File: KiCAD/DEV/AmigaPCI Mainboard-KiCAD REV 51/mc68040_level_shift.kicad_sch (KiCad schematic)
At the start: 27 parts, among them U231 74LVC08, U802 SN74LVC16T245DLR, U803 SN74LVC16T245DLR, U804 SN74LVC16T245DLR, U805 SN74LVC16T245DLR, U806 74LVC245, U807 74LVC245, U808 74LVC245, U809 74LVC245, U810 74LVC16646

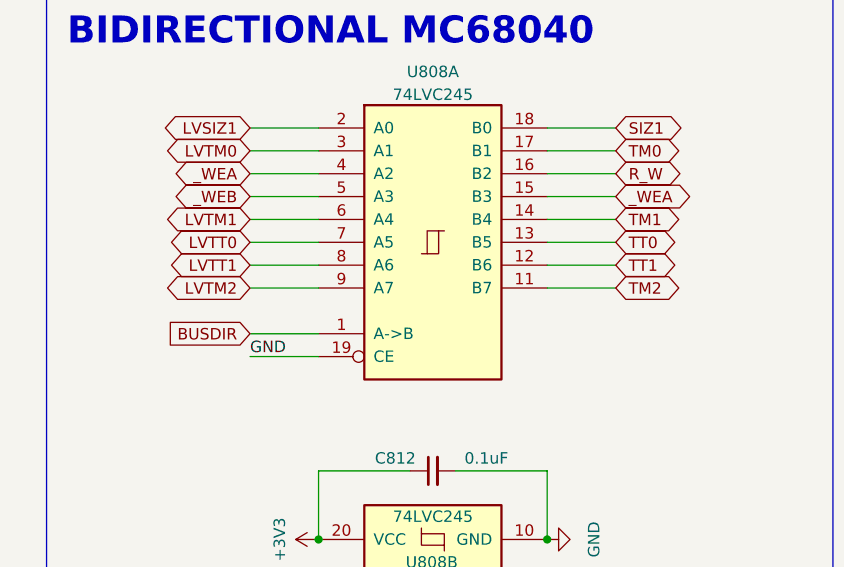
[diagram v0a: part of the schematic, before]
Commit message: Amiga PCI Rev 5.1 Work
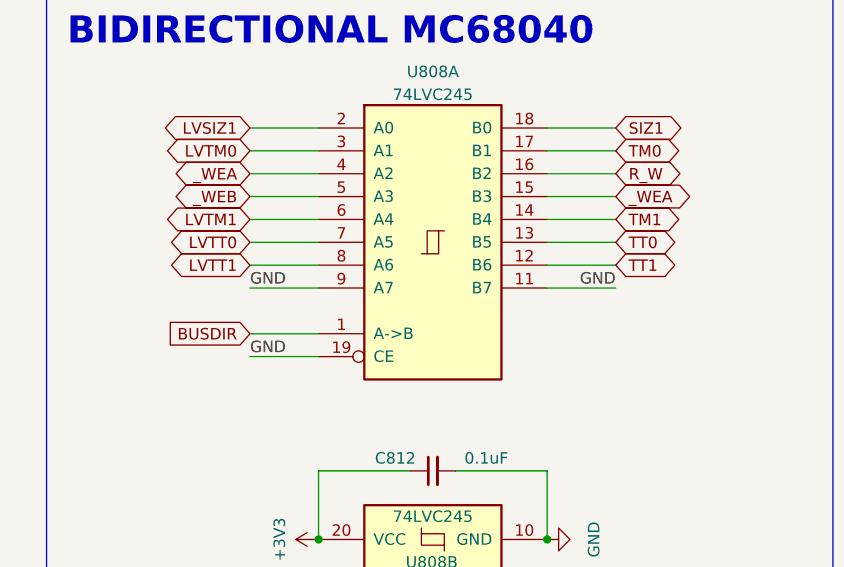
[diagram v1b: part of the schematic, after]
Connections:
- net LVTM2 is gone; now on net GND: U808.9 (A7)
- net TM2 is gone; now on net GND: U808.11 (B7)
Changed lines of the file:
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@@
 	(title_block
 		(title "AMIGA PCI")
-		(date "2025-03-31")
+		(date "2025-04-01")
 		(rev "5.1")
 	)
@@
 		)
 	)
+	(label "GND"
+		(at 234.95 170.18 0)
+		(effects
+			(font
+				(size 1.27 1.27)
+			)
+			(justify left bottom)
+		)
+	)
 	(label "UDB5"
 		(at 336.55 85.09 0)
@@
 		)
 	)
+	(label "GND"
+		(at 275.59 170.18 180)
+		(effects
+			(font
+				(size 1.27 1.27)
+			)
+			(justify right bottom)
+		)
+	)
 	(label "LVA29"
 		(at 120.65 157.48 0)
@@
 		)
 	)
-	(global_label "TM2"
-		(shape bidirectional)
-		(at 275.59 170.18 0)
-		(fields_autoplaced yes)
-		(effects
-			(font
-				(size 1.27 1.27)
-			)
-			(justify left)
-		)
-		(property "Intersheetrefs" "${INTERSHEET_REFS}"
-			(at 283.315 170.18 0)
-			(effects
-				(font
-					(size 1.27 1.27)
-				)
-				(justify left)
-			)
-		)
-	)
 	(global_label "DMALATCH"
 		(shape input)
@@
 			(effects
 				(font
-					(size 1.27 1.27)
-				)
-				(justify right)
-			)
-		)
-	)
-	(global_label "LVTM2"
-		(shape bidirectional)
-		(at 234.95 170.18 180)
-		(fields_autoplaced yes)
-		(effects
-			(font
-				(size 1.27 1.27)
-			)
-			(justify right)
-		)
-		(property "Intersheetrefs" "${INTERSHEET_REFS}"
-			(at 225.1083 170.18 0)
-			(effects
-				(font

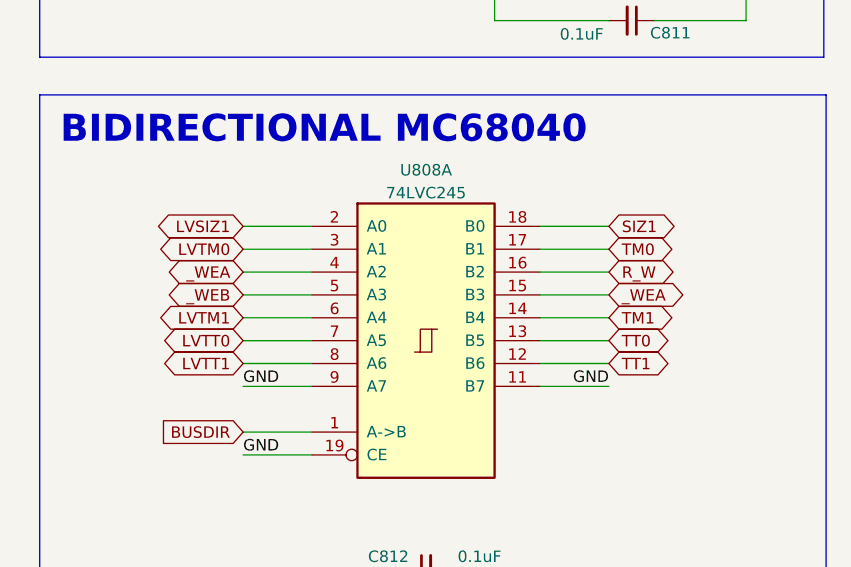
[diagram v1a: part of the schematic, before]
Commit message: APCI Rev 5.1 Work
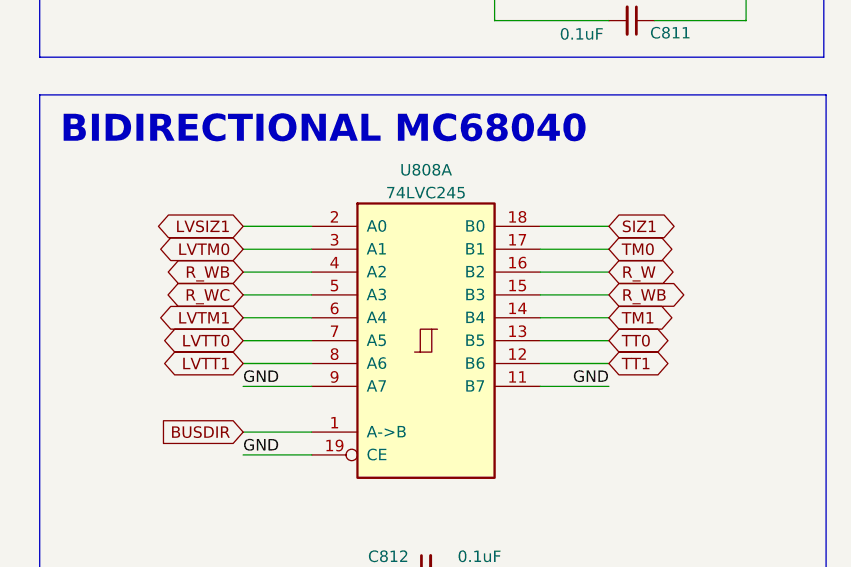
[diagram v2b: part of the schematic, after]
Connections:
- net _WEA renamed R_WB
- net _WEB renamed R_WC
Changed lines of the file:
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@@
 		)
 	)
-	(global_label "_WEB"
+	(global_label "R_WC"
 		(shape bidirectional)
 		(at 234.95 160.02 180)
@@
 		)
 	)
-	(global_label "_WEA"
+	(global_label "R_WB"
 		(shape bidirectional)
 		(at 275.59 160.02 0)
@@
 		)
 	)
-	(global_label "_WEA"
+	(global_label "R_WB"
 		(shape bidirectional)
 		(at 234.95 157.48 180)

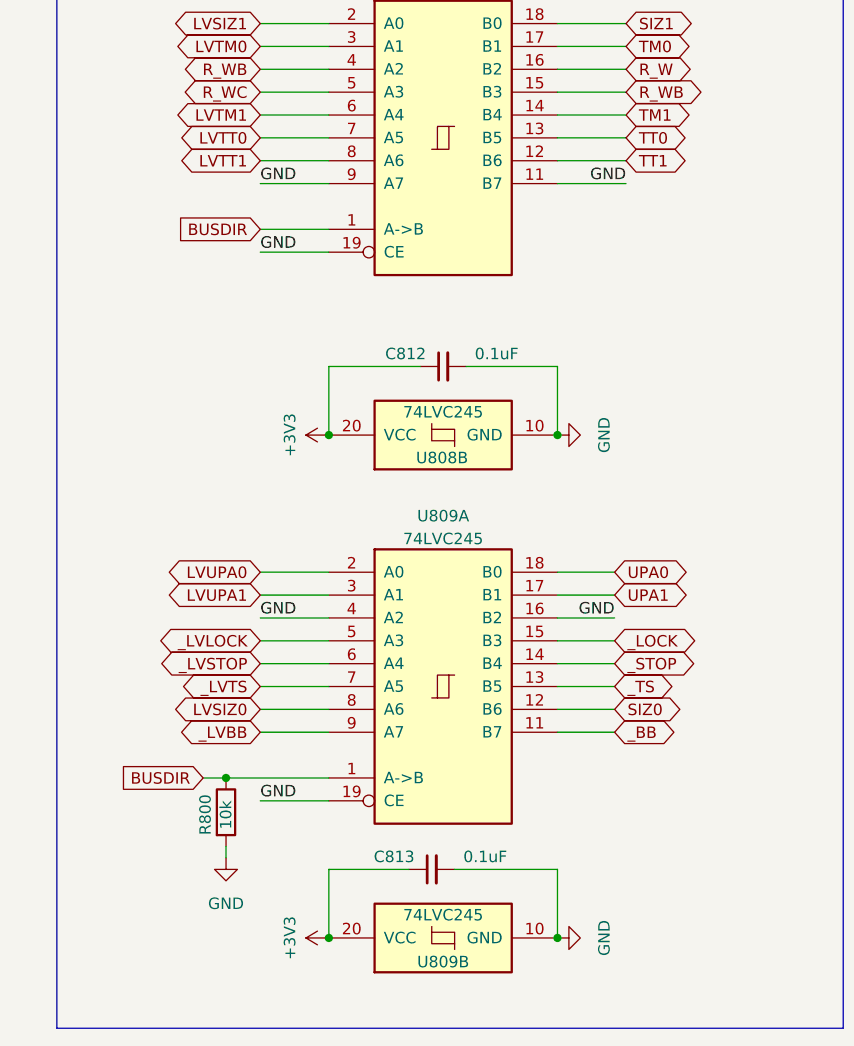
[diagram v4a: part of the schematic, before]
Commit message: APCI Rev 5.1 Work
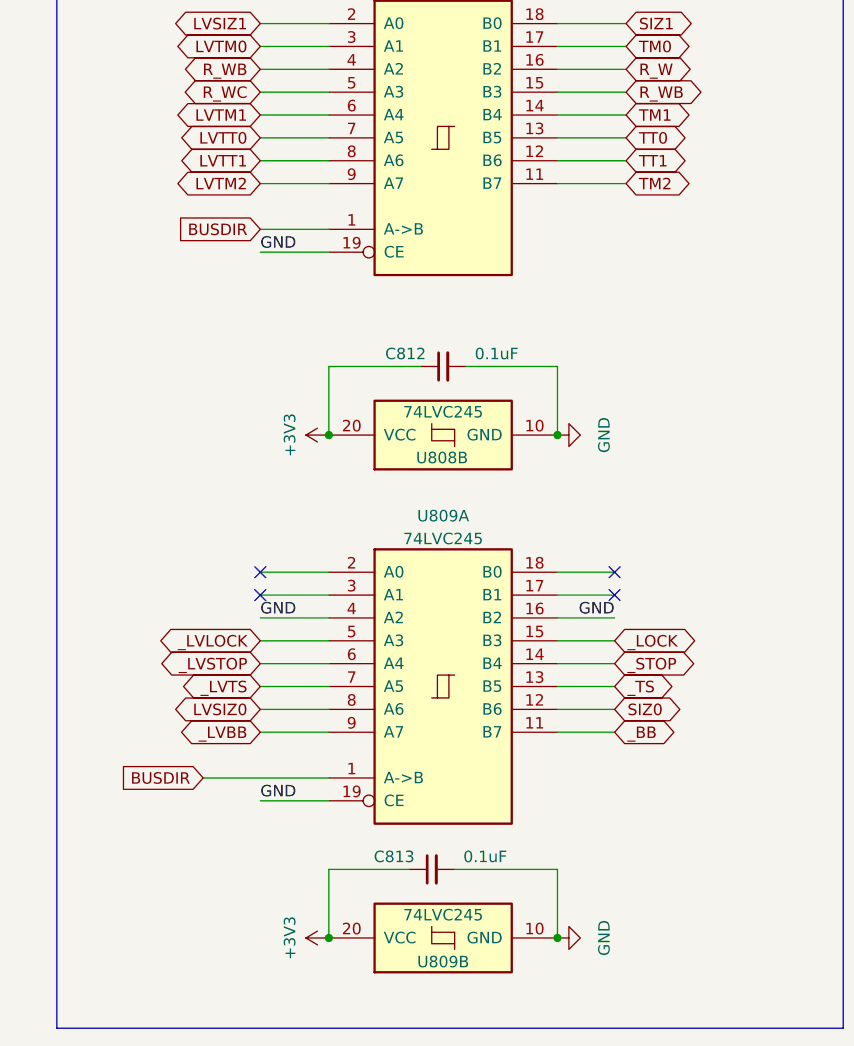
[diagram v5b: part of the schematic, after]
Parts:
- removed R800: 10k, Resistor_SMD:R_0603_1608Metric, symbol Device:R
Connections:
- net GND: no longer U808.11 (B7), U808.9 (A7)
- net LVUPA0: no longer names the net of U809.2 (A0)
- net LVUPA1: no longer names the net of U809.3 (A1)
- net UPA0: no longer names the net of U809.18 (B0)
- net UPA1: no longer names the net of U809.17 (B1)
- new net LVTM2: U808.9 (A7)
- new net TM2: U808.11 (B7)
- no-connect marks 0 -> 4
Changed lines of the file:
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@@
 	(title_block
 		(title "AMIGA PCI")
-		(date "2025-04-07")
+		(date "2025-04-10")
 		(rev "5.1")
 	)
@@
 	)
 	(junction
-		(at 231.14 236.22)
-		(diameter 0)
-		(color 0 0 0 0)
-	)
-	(junction
 		(at 267.97 254)
 		(diameter 0)
@@
 		(color 0 0 0 0)
 	)
+	(no_connect
+		(at 274.32 213.36)
+	)
+	(no_connect
+		(at 234.95 215.9)
+	)
+	(no_connect
+		(at 274.32 215.9)
+	)
+	(no_connect
+		(at 234.95 213.36)
+	)
 	(bus_entry
 		(at 120.65 129.54)
@@
 	(wire
 		(pts
-			(xy 242.57 236.22) (xy 231.14 236.22)
+			(xy 228.6 236.22) (xy 242.57 236.22)
 		)
 		(stroke
@@
 	(wire
 		(pts
-			(xy 231.14 243.84) (xy 231.14 245.11)
-		)
-		(stroke
-			(width 0)
-			(type default)
-		)
-	)
-	(wire
-		(pts
 			(xy 389.89 77.47) (xy 401.32 77.47)
 		)
@@
 	(wire
 		(pts
-			(xy 231.14 236.22) (xy 228.6 236.22)
-		)
-		(stroke
-			(width 0)
-			(type default)
-		)
-	)
-	(wire
-		(pts
 			(xy 31.75 191.77) (xy 93.98 191.77)
 		)
@@
 		)
 	)
-	(label "GND"
-		(at 234.95 170.18 0)
-		(effects
-			(font
-				(size 1.27 1.27)
-			)
-			(justify left bottom)
-		)
-	)
 	(label "UDB5"
 		(at 336.55 85.09 0)
@@
 		)
 	)
-	(label "GND"
-		(at 275.59 170.18 180)
-		(effects
-			(font
-				(size 1.27 1.27)
-			)
-			(justify right bottom)
-		)
-	)
 	(label "LVA29"
 		(at 120.65 157.48 0)
@@
 		)
 	)
-	(global_label "UPA1"
-		(shape bidirectional)
-		(at 274.32 215.9 0)
-		(fields_autoplaced yes)
-		(effects
-			(font
-				(size 1.27 1.27)
-			)
-			(justify left)
-		)
-		(property "Intersheetrefs" "${INTERSHEET_REFS}"
-			(at 283.3151 215.9 0)
-			(effects
-				(font
-					(size 1.27 1.27)
-				)
-				(justify left)
-			)
-		)
-	)
 	(global_label "LVTM0"
 		(shape bidirectional)
@@
 		)
 	)
-	(global_label "LVUPA0"
-		(shape bidirectional)
-		(at 234.95 213.36 180)
-		(fields_autoplaced yes)
-		(effects
-			(font
-				(size 1.27 1.27)
-			)
-			(justify right)
-		)
-		(property "Intersheetrefs" "${INTERSHEET_REFS}"
-			(at 223.8382 213.36 0)
-			(effects
-				(font
-					(size 1.27 1.27)
-				)
-				(justify right)
-			)
-		)
-	)
 	(global_label "UDB[15..0]"
 		(shape bidirectional)
@@
 		)
 	)
-	(global_label "UPA0"
-		(shape bidirectional)
-		(at 274.32 213.36 0)
-		(fields_autoplaced yes)
-		(effects
-			(font
-				(size 1.27 1.27)
-			)
-			(justify left)
-		)
-		(property "Intersheetrefs" "${INTERSHEET_REFS}"
-			(at 283.3151 213.36 0)
-			(effects
-				(font
-					(size 1.27 1.27)
-				)
-				(justify left)
-			)
-		)
-	)
 	(global_label "DRA1-0"
 		(shape input)
@@
 		)
 	)
-	(global_label "LVUPA1"
-		(shape bidirectional)
-		(at 234.95 215.9 180)
-		(fields_autoplaced yes)
-		(effects
-			(font
-				(size 1.27 1.27)
-			)
-			(justify right)
-		)
-		(property "Intersheetrefs" "${INTERSHEET_REFS}"
-			(at 223.8382 215.9 0)
-			(effects
-				(font
-					(size 1.27 1.27)
-				)
-				(justify right)
-			)
-		)
-	)
 	(global_label "D[31..0]"
 		(shape bidirectional)
@@
 		)
 	)
+	(global_label "TM2"
+		(shape bidirectional)
+		(at 275.59 170.18 0)
+		(fields_autoplaced yes)
+		(effects
+			(font
+				(size 1.27 1.27)
+			)
+			(justify left)
+		)
+		(property "Intersheetrefs" "${INTERSHEET_REFS}"
+			(at 283.315 170.18 0)
+			(effects
+				(font
+					(size 1.27 1.27)
+				)
+				(justify left)
+			)
+		)
+	)
+	(global_label "LVTM2"
+		(shape bidirectional)
+		(at 234.95 170.18 180)
+		(fields_autoplaced yes)
+		(effects
+			(font
+				(size 1.27 1.27)
+			)
+			(justify right)
+		)
+		(property "Intersheetrefs" "${INTERSHEET_REFS}"
+			(at 225.1083 170.18 0)
+			(effects
+				(font
+					(size 1.27 1.27)
+				)
+				(justify right)
+			)
+		)
+	)
 	(global_label "LVDRA8-7"
 		(shape output)
@@
 		(shape input)
 		(at 228.6 236.22 180)
-		(fields_autoplaced yes)
 		(effects
 			(font
@@
 		)
 		(property "Intersheetrefs" "${INTERSHEET_REFS}"
-			(at 218.66 236.22 0)
+			(at 220.218 236.22 0)
 			(effects
 				(font
@@
 	)
 	(symbol
-		(lib_id "Device:R")
-		(at 231.14 240.03 0)
-		(unit 1)
-		(exclude_from_sim no)
-		(in_bom yes)
-		(on_board yes)
-		(dnp no)
-		(property "Reference" "R800"
-			(at 228.854 242.57 90)
-			(effects
-				(font
-					(size 1.27 1.27)
-				)
-				(justify left)
-			)
-		)
-		(property "Value" "10k"
-			(at 231.14 241.935 90)
-			(effects
-				(font
-					(size 1.27 1.27)
-				)
-				(justify left)
-			)
-		)
-		(property "Footprint" "Resistor_SMD:R_0603_1608Metric"
-			(at 229.362 240.03 90)
-			(effects
-				(font
-					(size 1.27 1.27)
-				)
-				(hide yes)
-			)
-		)
-		(property "Datasheet" "~"
-			(at 231.14 240.03 0)
-			(effects
-				(font
-					(size 1.27 1.27)
-				)
-				(hide yes)
-			)
-		)
-		(property "Description" ""
-			(at 231.14 240.03 0)
-			(effects
-				(font
-					(size 1.27 1.27)
-				)
-				(hide yes)
-			)
-		)
-		(pin "1"
-		)
-		(pin "2"
-		)
-		(instances
-			(project "AmigaPCI Mainboard"
-				(path "/72453515-27fe-4336-91f3-e3c8054f7767/3746f476-970c-4acb-b19d-33c43fff35fb"
-					(reference "R800")
-					(unit 1)
-				)
-			)
-		)
-	)
-	(symbol
 		(lib_id "AmigaPCI-Symbols:74LVC16646")
 		(at 369.57 88.9 0)
@@
 					(unit 1)
 				)
-			)
-		)
-	)
-	(symbol
-		(lib_id "power:GND")
-		(at 231.14 245.11 0)
-		(mirror y)
-		(unit 1)
-		(exclude_from_sim no)
-		(in_bom yes)
-		(on_board yes)
-		(dnp no)
-		(fields_autoplaced yes)
-		(property "Reference" "#PWR0199"
-			(at 231.14 251.46 0)
-			(effects
-				(font
-					(size 1.27 1.27)
-				)
-				(hide yes)
-			)
-		)
-		(property "Value" "GND"
-			(at 231.14 250.19 0)
-			(effects
-				(font
-					(size 1.27 1.27)
-				)
-			)
-		)
-		(property "Footprint" ""
-			(at 231.14 245.11 0)
-			(effects
-				(font
-					(size 1.27 1.27)
-				)
-				(hide yes)
-			)
-		)
-		(property "Datasheet" ""
-			(at 231.14 245.11 0)
-			(effects
-				(font
-					(size 1.27 1.27)
-				)
-				(hide yes)
-			)
-		)
-		(property "Description" ""
-			(at 231.14 245.11 0)
-			(effects
-				(font
-					(size 1.27 1.27)
-				)
-				(hide yes)
-			)
-		)
-		(pin "1"
-		)
-		(instances
-			(project "AmigaPCI Mainboard"
-				(path "/72453515-27fe-4336-91f3-e3c8054f7767/3746f476-970c-4acb-b19d-33c43fff35fb"
-					(reference "#PWR0199")
-					(unit 1)
-				)
